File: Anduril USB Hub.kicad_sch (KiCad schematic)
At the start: 30 parts, among them J1 USB C 2.0, Upstream, J2 USB A, Port 1, J3 USB A, Port 2, J4 USB C 2.0, Port 3, U1 USB4604-1080HN, U2 USBLC6-2SC6, U3 USBLC6-2SC6, U4 USBLC6-2SC6, Y1 Crystal_GND24

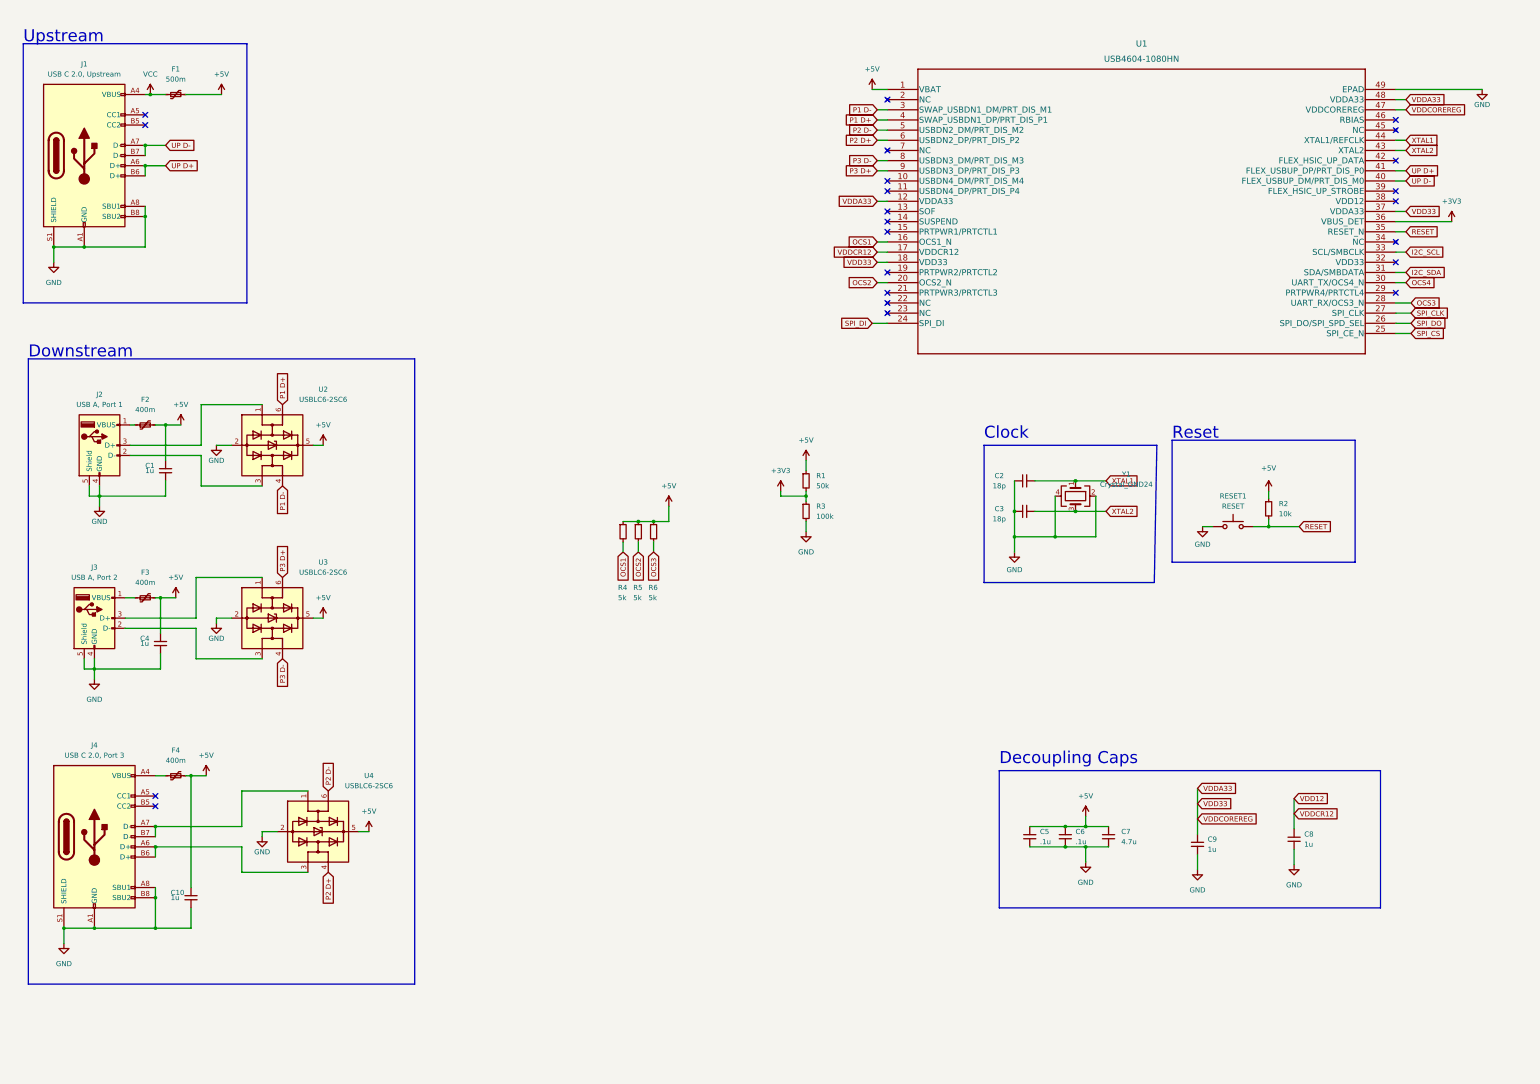
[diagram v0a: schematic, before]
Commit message: layout done, saving for 0805 change
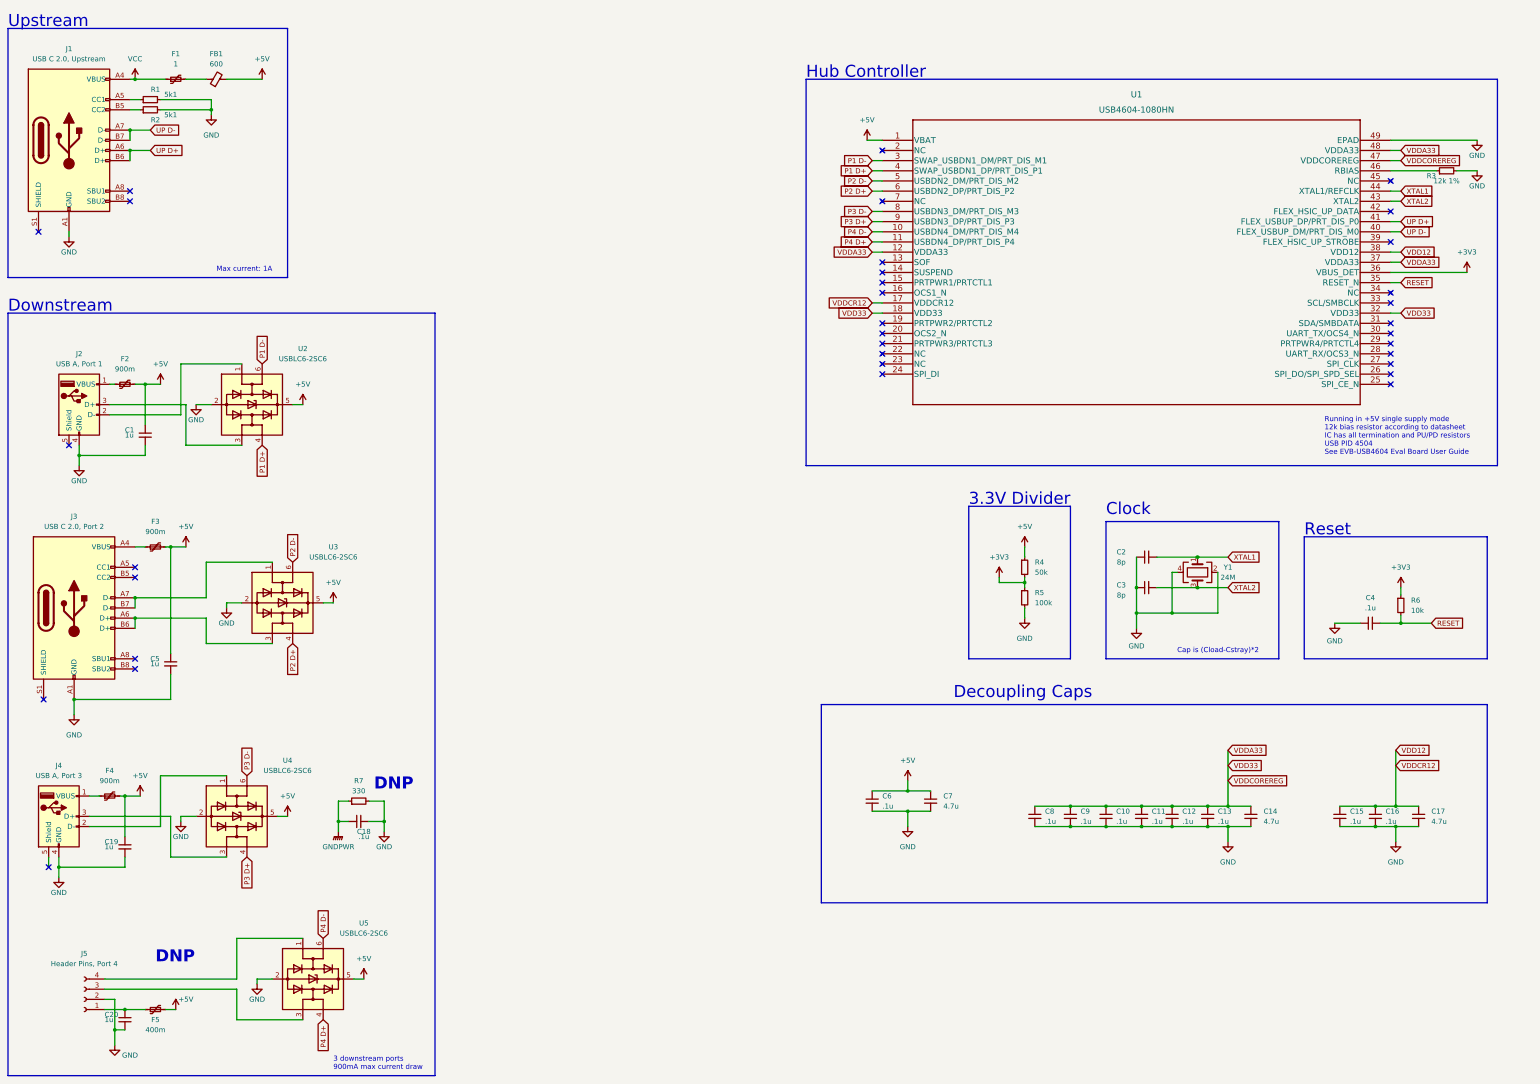
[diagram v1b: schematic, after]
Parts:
- removed C6: .1u, Capacitor_SMD:C_0805_2012Metric, symbol Device:C_Small
- removed R4, R5, R6: 5k, Resistor_SMD:R_0805_2012Metric, symbol Device:R_Small
- removed RESET1: RESET, colonDcustom:Pushbutton_TH_6x6, symbol Switch:SW_Push
- added C10, C11, C12, C13, C15, C16, C4: .1u, Capacitor_SMD:C_0402_1005Metric, symbol Device:C_Small
- added C14, C17: 4.7u, Capacitor_SMD:C_0603_1608Metric, symbol Device:C_Small
- added C18: .1u, Capacitor_SMD:C_0603_1608Metric, symbol Device:C_Small
- added C20: 1u, Capacitor_SMD:C_0603_1608Metric, symbol Device:C_Small
- added F5: 400m, Fuse:Fuse_0603_1608Metric, symbol Device:Polyfuse_Small
- added FB1: 600, Resistor_SMD:R_0603_1608Metric, symbol Device:FerriteBead_Small
- added J5: Header Pins, Port 4, Connector_PinHeader_1.27mm:PinHeader_1x04_P1.27mm_Horizontal, symbol Connector:Conn_01x04_Female
- added R1, R2: 5k1, Resistor_SMD:R_0603_1608Metric, symbol Device:R_Small
- added R3: 12k 1%, Resistor_SMD:R_0603_1608Metric, symbol Device:R_Small
- added R7: 330, Resistor_SMD:R_0603_1608Metric, symbol Device:R_Small
- added U5: USBLC6-2SC6, Package_TO_SOT_SMD:SOT-23-6, symbol Power_Protection:USBLC6-2SC6
- C1, C7: footprint Capacitor_SMD:C_0805_2012Metric -> Capacitor_SMD:C_0603_1608Metric
- C19: renamed from C4; footprint Capacitor_SMD:C_0805_2012Metric -> Capacitor_SMD:C_0603_1608Metric
- C2, C3: value 18p -> 8p; footprint Capacitor_SMD:C_0805_2012Metric -> Capacitor_SMD:C_0402_1005Metric
- C5: renamed from C10; footprint Capacitor_SMD:C_0805_2012Metric -> Capacitor_SMD:C_0603_1608Metric
- C6: renamed from C5; footprint Capacitor_SMD:C_0805_2012Metric -> Capacitor_SMD:C_0402_1005Metric
- C8, C9: value 1u -> .1u; footprint Capacitor_SMD:C_0805_2012Metric -> Capacitor_SMD:C_0402_1005Metric
- F1: value 500m -> 1; footprint Fuse:Fuse_0805_2012Metric -> Fuse:Fuse_0603_1608Metric
- F2: value 400m -> 900m; footprint Fuse:Fuse_0805_2012Metric -> Fuse:Fuse_0603_1608Metric
- F3: renamed from F4; value 400m -> 900m; footprint Fuse:Fuse_0805_2012Metric -> Fuse:Fuse_0603_1608Metric
- F4: renamed from F3; value 400m -> 900m; footprint Fuse:Fuse_0805_2012Metric -> Fuse:Fuse_0603_1608Metric
- J1: footprint Connector_USB:USB_C_Receptacle_GCT_USB4085 -> colonDcustom:USB_C_Receptacle_HRO_TYPE-C-31-M-12
- J2: footprint Connector_USB:USB3_A_Molex_48393-001 -> colonDcustom:USB_A_CONNFLY_DS1095-WNR0
- J3: renamed from J4; value USB C 2.0, Port 3 -> USB C 2.0, Port 2; footprint Connector_USB:USB_C_Receptacle_GCT_USB4085 -> colonDcustom:USB_C_Receptacle_HRO_TYPE-C-31-M-12
- J4: renamed from J3; value USB A, Port 2 -> USB A, Port 3; footprint Connector_USB:USB3_A_Molex_48393-001 -> colonDcustom:USB_A_CONNFLY_DS1095-WNR0
- R4: renamed from R1; footprint Resistor_SMD:R_0805_2012Metric -> Resistor_SMD:R_0603_1608Metric
- R5: renamed from R3; footprint Resistor_SMD:R_0805_2012Metric -> Resistor_SMD:R_0603_1608Metric
- R6: renamed from R2; footprint Resistor_SMD:R_0805_2012Metric -> Resistor_SMD:R_0603_1608Metric
- Y1: value Crystal_GND24 -> 24M; footprint Crystal:Crystal_SMD_0603-4Pin_6.0x3.5mm -> Crystal:Crystal_SMD_2016-4Pin_2.0x1.6mm
- renumbered U4 to U3, U3 to U4
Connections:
- net +3V3: now also R6.1
- net +5V: now also F5.2, FB1.2, U5.5 (VBUS); no longer F1.2, R6.1
- net GND: now also C10.2, C11.2, C12.2, C13.2, C14.2, C15.2, C16.2, C17.2, C18.2, C20.2, C4.1, J5.2 (Pin_2), R1.2, R2.2, R3.2, R7.2, U5.2 (GND); no longer J1.A8 (SBU1), J1.B8 (SBU2), J1.S1 (SHIELD), J2.5 (Shield), J3.A8 (SBU1), J3.B8 (SBU2), J3.S1 (SHIELD), J4.5 (Shield)
- net P1 D+: now also U2.4 (I/O2); no longer U2.6 (I/O1)
- net P1 D-: now also U2.6 (I/O1); no longer U2.4 (I/O2)
- net P3 D+: now also U4.4 (I/O2); no longer U4.6 (I/O1)
- net P3 D-: now also U4.6 (I/O1); no longer U4.4 (I/O2)
- net RESET: now also C4.2
- net VDD12: now also U1.38 (VDD12), C15.1, C16.1, C17.1; no longer C8.1
- net VDD33: now also C8.1, U1.32 (VDD33), C10.1, C11.1, C12.1, C13.1, C14.1
- net at J4.2 (D-): now also U4.1 (I/O1); no longer U4.3 (I/O2)
- net at J4.3 (D+): now also U4.3 (I/O2); no longer U4.1 (I/O1)
- net P4 D-: now reaches U1.10 (USBDN4_DM/PRT_DIS_M4)
- net P4 D-: now also U5.6 (I/O1)
- net P4 D+: now reaches U1.11 (USBDN4_DP/PRT_DIS_P4)
- net P4 D+: now also U5.4 (I/O2)
- net at U1.46 (RBIAS): now also R3.1
- net at J1.A5 (CC1): now also R1.1
- net at J1.B5 (CC2): now also R2.1
- net at J2.2 (D-): now also U2.1 (I/O1); no longer U2.3 (I/O2)
- net at J2.3 (D+): now also U2.3 (I/O2); no longer U2.1 (I/O1)
- net I2C_SCL: no longer names the net of U1.33 (SCL/SMBCLK)
- net I2C_SDA: no longer names the net of U1.31 (SDA/SMBDATA)
- net OCS1: no longer names the net of U1.16 (OCS1_N)
- net OCS2: no longer names the net of U1.20 (OCS2_N)
- net OCS3: no longer names the net of U1.28 (UART_RX/OCS3_N)
- net OCS4: no longer names the net of U1.30 (UART_TX/OCS4_N)
- net SPI_CLK: no longer names the net of U1.27 (SPI_CLK)
- net SPI_CS: no longer names the net of U1.25 (SPI_CE_N)
- net SPI_DI: no longer names the net of U1.24 (SPI_DI)
- net SPI_DO: no longer names the net of U1.26 (SPI_DO/SPI_SPD_SEL)
- new net: C20.1, F5.1, J5.1 (Pin_1)
- new net: J5.3 (Pin_3), U5.3 (I/O2)
- new net: J5.4 (Pin_4), U5.1 (I/O1)
- new net: F1.2, FB1.1
- new net GNDPWR: C18.1, R7.1
- no-connect marks 23 -> 34
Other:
- note added: "3 downstream ports 900mA max current draw"
- note added: "3.3V Divider"
- note added: "Cap is (Cload-Cstray)*2"
- note added: "DNP"
- note added: "Hub Controller"
- note added: "Max current: 1A"
- note added: "Running in +5V single supply mode 12k bias resistor according to datasheet IC has all termination and PU/PD resistors USB PID 4504 See EVB-USB4604 Eval Board User Guide"
- moved on the sheet: C1, C19, C2, C3, C5, C6, C7, F1, F2, F3, F4, J1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

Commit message: V1.0
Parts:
- C1, C14, C17, C19, C5, C7: footprint Capacitor_SMD:C_0603_1608Metric -> Capacitor_SMD:C_0805_2012Metric
- C10, C11, C12, C13, C15, C16, C2, C3, C4, C6, C8, C9: footprint Capacitor_SMD:C_0402_1005Metric -> Capacitor_SMD:C_0805_2012Metric
- F1, F2, F3, F4: footprint Fuse:Fuse_0603_1608Metric -> Fuse:Fuse_0805_2012Metric
- FB1, R1, R2, R3, R4, R5, R6: footprint Resistor_SMD:R_0603_1608Metric -> Resistor_SMD:R_0805_2012Metric
- Y1: footprint Crystal:Crystal_SMD_2016-4Pin_2.0x1.6mm -> Crystal:Crystal_SMD_3225-4Pin_3.2x2.5mm
